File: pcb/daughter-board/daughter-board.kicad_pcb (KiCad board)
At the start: 2 copper layers, 50 x 30 mm, 11 parts, among them J1 Conn_01x06_MountingPin, J2 USB_C_Receptacle_USB2.0_16P, J4 4P4C_Shielded, U1 SRV05-4

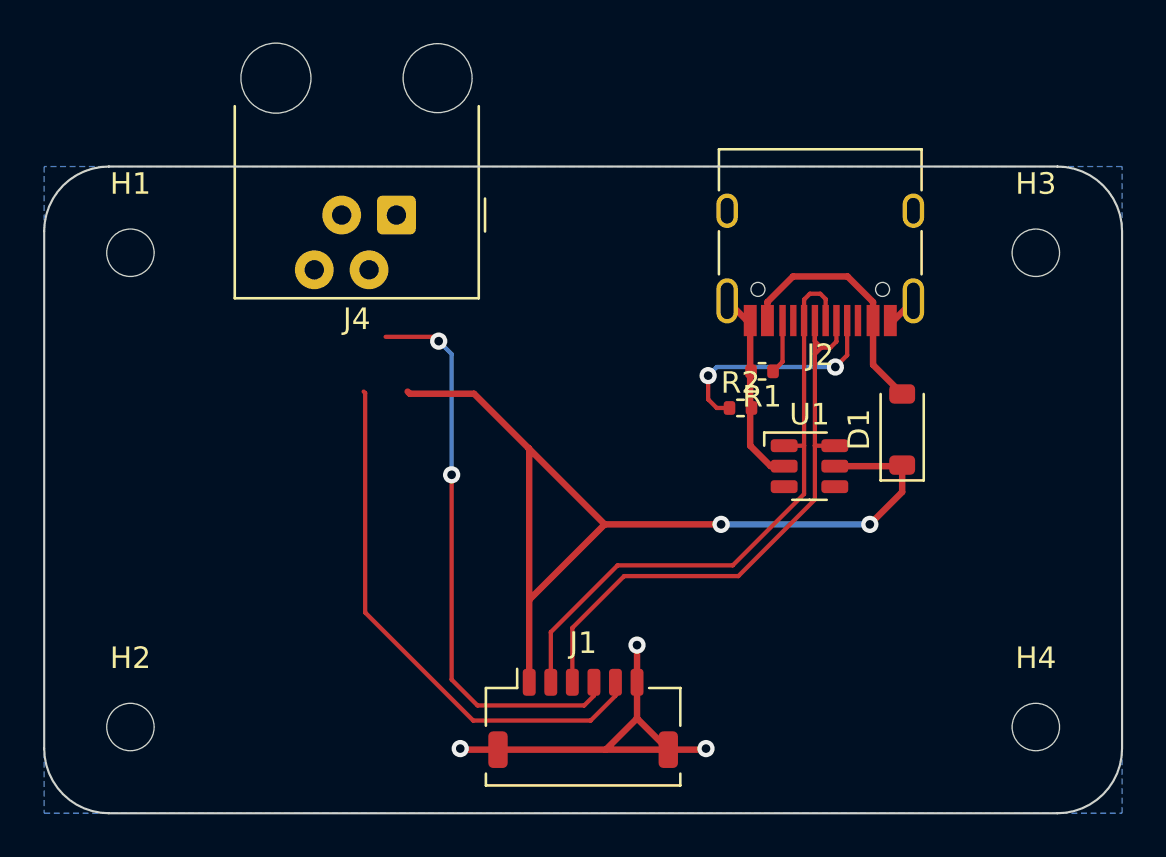
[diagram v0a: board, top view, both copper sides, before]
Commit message: schematics review with scgh
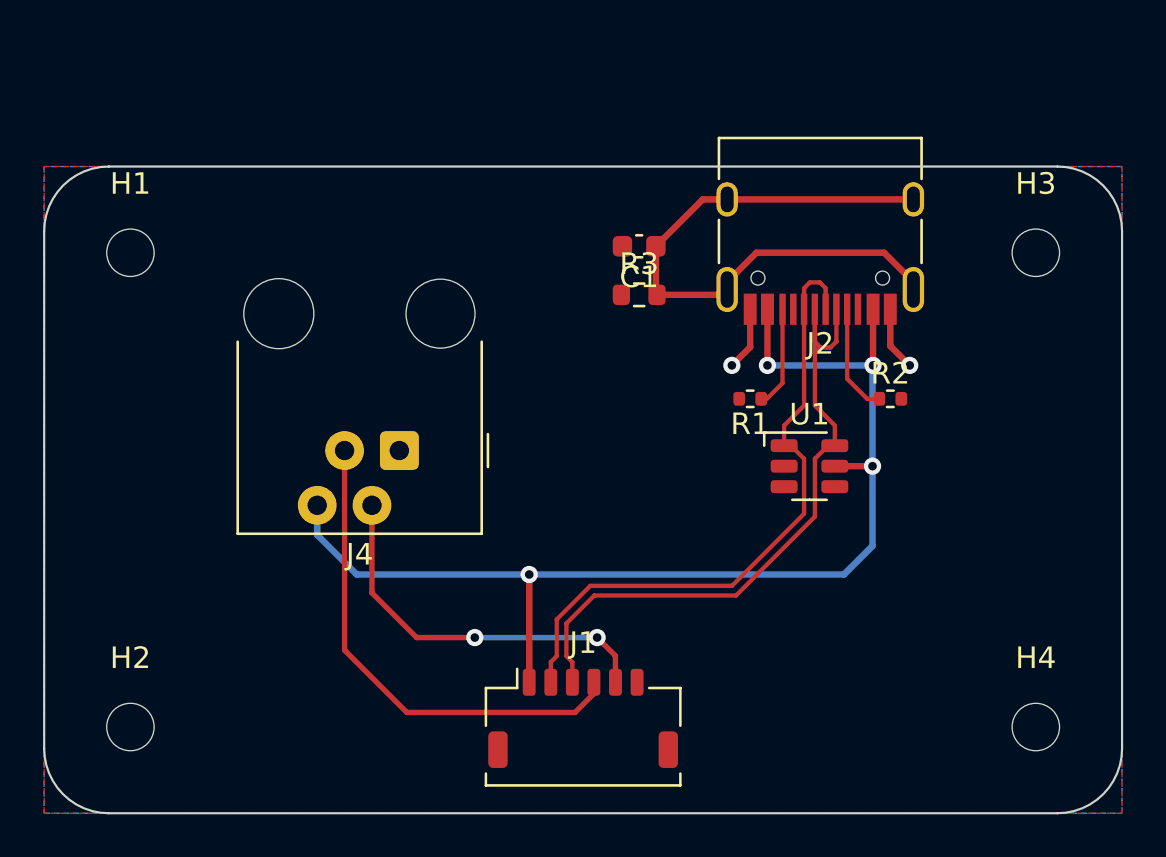
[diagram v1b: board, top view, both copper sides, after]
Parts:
- removed D1: D_Schottky, Diode_SMD:D_SOD-123
- added C1: 100n, Capacitor_SMD:C_0603_1608Metric, F.Cu at (127.6, 63.7)
- added R3: 220k, Resistor_SMD:R_0603_1608Metric, F.Cu at (127.6, 66.0)
- moved J4 10.9 mm to (116.5, 73.2)
- moved R2 6.96 mm to (139.2, 70.8)
- moved R1 1.39 mm to (132.8, 70.8)
- moved J2 0.52 mm to (136.0, 62.6)
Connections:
- J2 pad A4: VBUS -> +5V
- J2 pad A9: VBUS -> +5V
- J2 pad B4: VBUS -> +5V
- J2 pad B9: VBUS -> +5V
- J2 pad S1: GND -> Net-(J2-SHIELD)
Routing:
- net Net-(J2-SHIELD): track 0.00 -> 28.9 mm
- net GND: track 29.7 -> 5.93 mm, vias 3 -> 2
- net VBUS: track 11.6 -> 0.00 mm
- net +5V: track 46.4 -> 53.7 mm, vias 2 -> 4
- net /SPLIT_RX: track 25.1 -> 17.8 mm, vias 0 -> 2
- net Net-(J2-CC1): track 10.7 -> 5.10 mm, vias 2 -> 0
- net /SPLIT_TX: track 26.4 -> 22.9 mm, vias 2 -> 0
- net /USB_D-: track 29.1 -> 31.6 mm
- net Net-(J2-CC2): track 2.54 -> 4.72 mm
- net /USB_D+: track 28.9 -> 30.1 mm
- added copper zone on F.Cu, net GND
